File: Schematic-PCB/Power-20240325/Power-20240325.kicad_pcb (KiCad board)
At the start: 2 copper layers, 43.9 x 82.2 mm, 0 parts

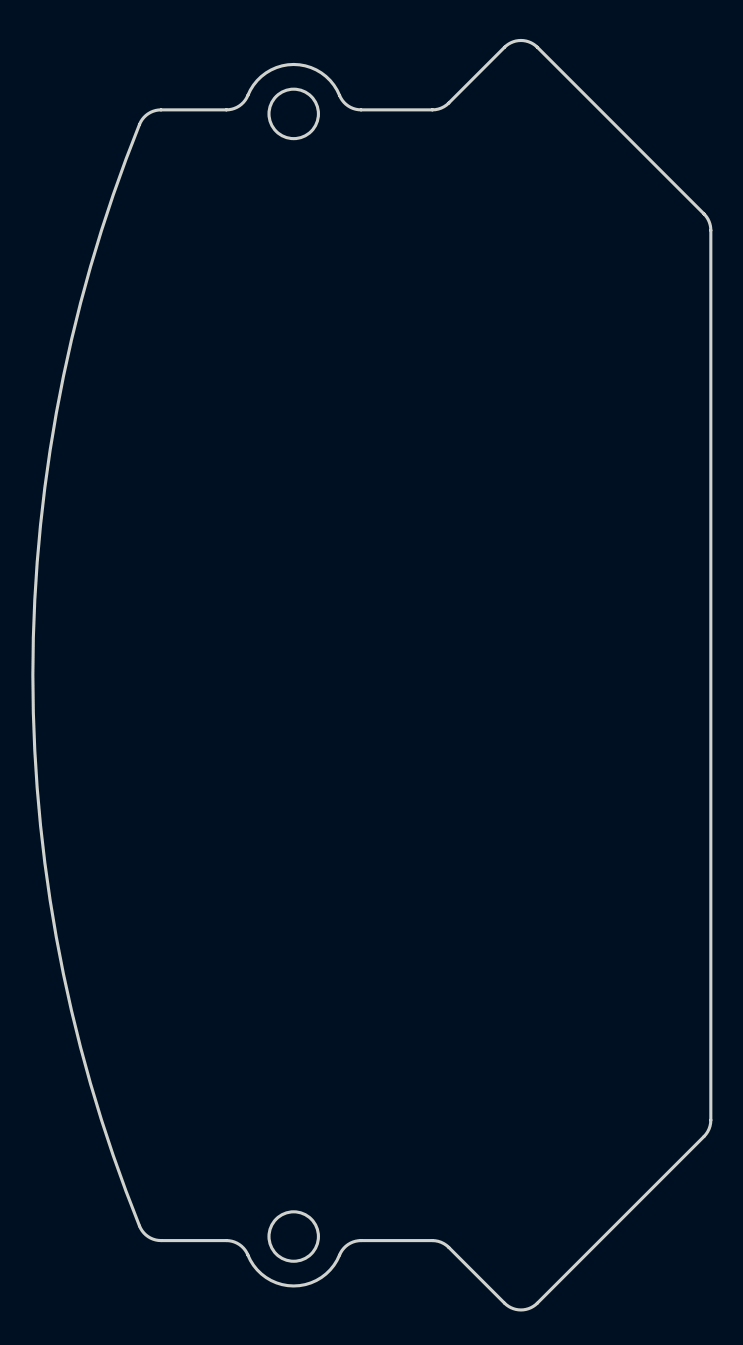
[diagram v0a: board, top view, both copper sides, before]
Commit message: MD基板の仮完成
DRをお願いします
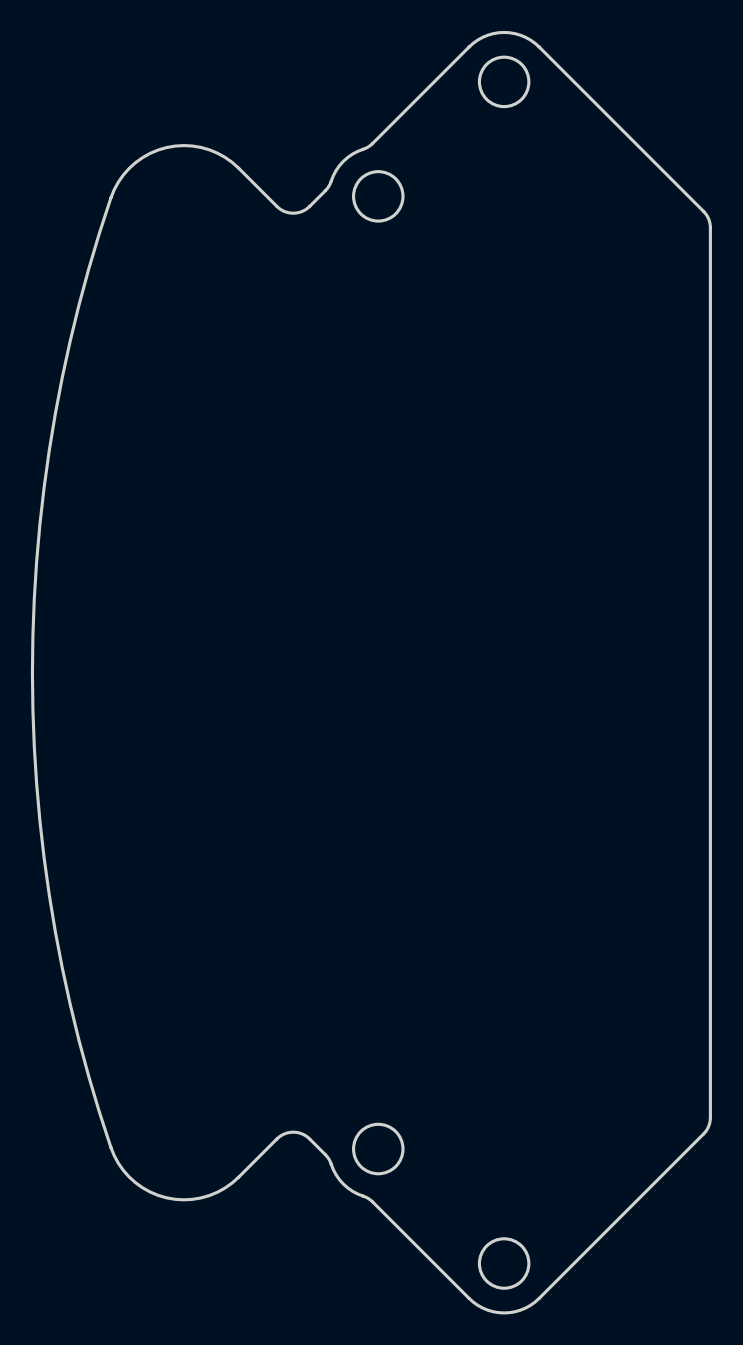
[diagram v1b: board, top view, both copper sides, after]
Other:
- board size 43.9 x 82.2 mm -> 43.9 x 82.9 mm
